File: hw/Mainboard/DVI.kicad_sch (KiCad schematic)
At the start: 15 parts, among them J23 NOT_HDMI_A

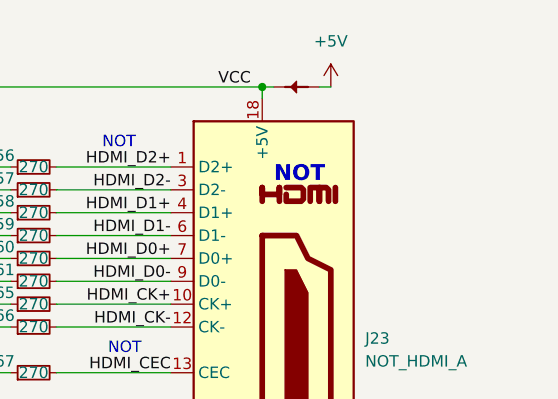
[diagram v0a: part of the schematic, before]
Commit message: hw: caps & logos (wip)
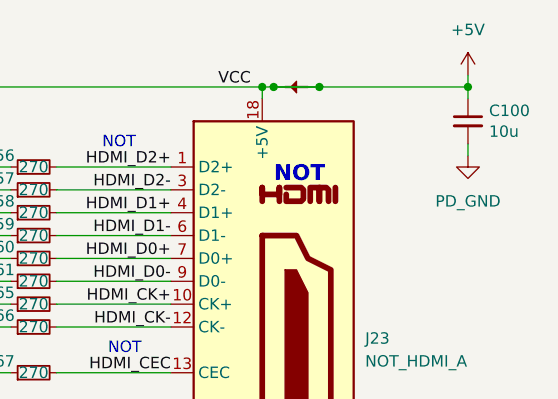
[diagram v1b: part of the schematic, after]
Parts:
- added C100: 10u, Capacitor_SMD:C_0603_1608Metric, symbol Device:C_Small
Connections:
- net VCC is gone; now on net +5V: J23.18 (+5V), PT49.2, R63.1, R64.1
- net +5V: now also C100.1
- net PD_GND: now also C100.2
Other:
- title: CBM PET Mainboard Replacement -> EconoPET 40/8096
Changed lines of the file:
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@@
   (paper "A")
   (title_block
-    (title "CBM PET Mainboard Replacement")
+    (title "EconoPET 40/8096")
+    (date "2023-10-01")
+    (rev "A")
   )
   (bus_alias "DVI" (members "DVI_D2+" "DVI_D2-" "DVI_D1+" "DVI_D1-" "DVI_D0+" "DVI_D0-" "DVI_CK+" "DVI_CK-"))
   (junction (at 134.62 111.76) (diameter 0) (color 0 0 0 0)
   )
+  (junction (at 196.85 59.69) (diameter 0) (color 0 0 0 0)
+  )
   (junction (at 193.04 120.65) (diameter 0) (color 0 0 0 0)
   )
+  (junction (at 213.36 59.69) (diameter 0) (color 0 0 0 0)
+  )
   (junction (at 193.04 118.11) (diameter 0) (color 0 0 0 0)
   )
   (junction (at 190.5 59.69) (diameter 0) (color 0 0 0 0)
+  )
+  (junction (at 191.77 59.69) (diameter 0) (color 0 0 0 0)
   )
   (junction (at 134.62 59.69) (diameter 0) (color 0 0 0 0)
@@
     (stroke (width 0) (type default) (color 0 0 0 0))
   )
+  (wire (pts (xy 213.36 67.31) (xy 213.36 66.04))
+    (stroke (width 0) (type default) (color 0 0 0 0))
+  )
   (bus (pts (xy 146.05 71.12) (xy 146.05 73.66))
     (stroke (width 0) (type default) (color 0 0 0 0))
@@
     (stroke (width 0) (type default) (color 0 0 0 0))
   )
+  (wire (pts (xy 196.85 59.69) (xy 213.36 59.69))
+    (stroke (width 0) (type default) (color 0 0 0 0))
+  )
   (wire (pts (xy 167.64 68.58) (xy 180.34 68.58))
     (stroke (width 0) (type default) (color 0 0 0 0))
@@
     (stroke (width 0) (type default) (color 0 0 0 0))
   )
+  (wire (pts (xy 213.36 59.69) (xy 213.36 58.42))
+    (stroke (width 0) (type default) (color 0 0 0 0))
+  )
   (wire (pts (xy 190.5 59.69) (xy 190.5 60.96))
     (stroke (width 0) (type default) (color 0 0 0 0))
@@
     (stroke (width 0) (type default) (color 0 0 0 0))
   )
+  (wire (pts (xy 213.36 60.96) (xy 213.36 59.69))
+    (stroke (width 0) (type default) (color 0 0 0 0))
+  )
+  (wire (pts (xy 191.77 59.69) (xy 196.85 59.69))
+    (stroke (width 0) (type default) (color 0 0 0 0))
+  )
   (wire (pts (xy 193.04 120.65) (xy 198.12 120.65))
     (stroke (width 0) (type default) (color 0 0 0 0))
@@
   )
   (wire (pts (xy 129.54 101.6) (xy 163.83 101.6))
-    (stroke (width 0) (type default) (color 0 0 0 0))
-  )
-  (wire (pts (xy 198.12 59.69) (xy 196.85 59.69))
     (stroke (width 0) (type default) (color 0 0 0 0))
   )
@@
     (pin "2")
   )
-  (symbol (lib_id "power:+5V") (at 198.12 59.69 0) (unit 1)
+  (symbol (lib_id "power:+5V") (at 213.36 58.42 0) (unit 1)
     (in_bom yes) (on_board yes) (fields_autoplaced)
-    (property "Reference" "#PWR0149" (id 0) (at 198.12 63.5 0)
-      (effects (font (size 1.27 1.27)) hide)
-    )
-    (property "Value" "+5V" (id 1) (at 198.12 54.61 0))
-    (property "Footprint" "" (id 2) (at 198.12 59.69 0)
-      (effects (font (size 1.27 1.27)) hide)
-    )
-    (property "Datasheet" "" (id 3) (at 198.12 59.69 0)
+    (property "Reference" "#PWR0149" (id 0) (at 213.36 62.23 0)
+      (effects (font (size 1.27 1.27)) hide)
+    )
+    (property "Value" "+5V" (id 1) (at 213.36 53.34 0))
+    (property "Footprint" "" (id 2) (at 213.36 58.42 0)
+      (effects (font (size 1.27 1.27)) hide)
+    )
+    (property "Datasheet" "" (id 3) (at 213.36 58.42 0)
       (effects (font (size 1.27 1.27)) hide)
     )
@@
     (pin "2")
   )
+  (symbol (lib_id "Device:C_Small") (at 213.36 63.5 0) (unit 1)
+    (in_bom yes) (on_board yes)
+    (property "Reference" "C100" (id 0) (at 215.6968 62.3316 0)
+      (effects (font (size 1.27 1.27)) (justify left))
+    )
+    (property "Value" "10u" (id 1) (at 215.6968 64.643 0)
+      (effects (font (size 1.27 1.27)) (justify left))
+    )
+    (property "Footprint" "Capacitor_SMD:C_0603_1608Metric" (id 2) (at 213.36 63.5 0)
+      (effects (font (size 1.27 1.27)) hide)
+    )
+    (property "Datasheet" "https://datasheet.lcsc.com/lcsc/2304140030_Samsung-Electro-Mechanics-CL10A106MA8NRNC_C96446.pdf" (id 3) (at 213.36 63.5 0)
+      (effects (font (size 1.27 1.27)) hide)
+    )
+    (property "LCSC" "C96446" (id 4) (at 213.36 63.5 0)
+      (effects (font (size 1.27 1.27)) hide)
+    )
+    (pin "1")
+    (pin "2")
+  )
   (symbol (lib_id "Device:R_Small") (at 165.1 78.74 90) (unit 1)
     (in_bom yes) (on_board yes)
@@
     (pin "2")
   )
+  (symbol (lib_id "PET:PD_GND") (at 213.36 67.31 0) (unit 1)
+    (in_bom yes) (on_board yes) (fields_autoplaced)
+    (property "Reference" "#PWR0176" (id 0) (at 213.36 73.66 0)
+      (effects (font (size 1.27 1.27)) hide)
+    )
+    (property "Value" "PD_GND" (id 1) (at 213.36 72.39 0))
+    (property "Footprint" "" (id 2) (at 213.36 67.31 0)
+      (effects (font (size 1.27 1.27)) hide)
+    )
+    (property "Datasheet" "" (id 3) (at 213.36 67.31 0)
+      (effects (font (size 1.27 1.27)) hide)
+    )
+    (pin "1")
+  )
 )
